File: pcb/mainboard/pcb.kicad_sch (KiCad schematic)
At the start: 28 parts

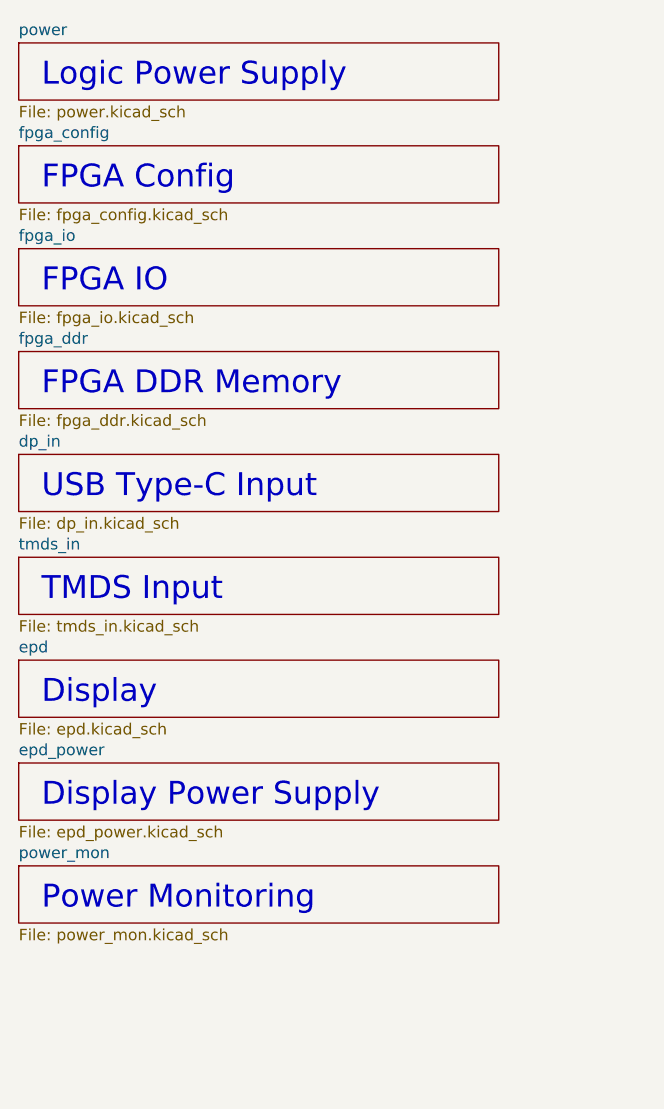
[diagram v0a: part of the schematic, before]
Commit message: PCB r0p10 wip
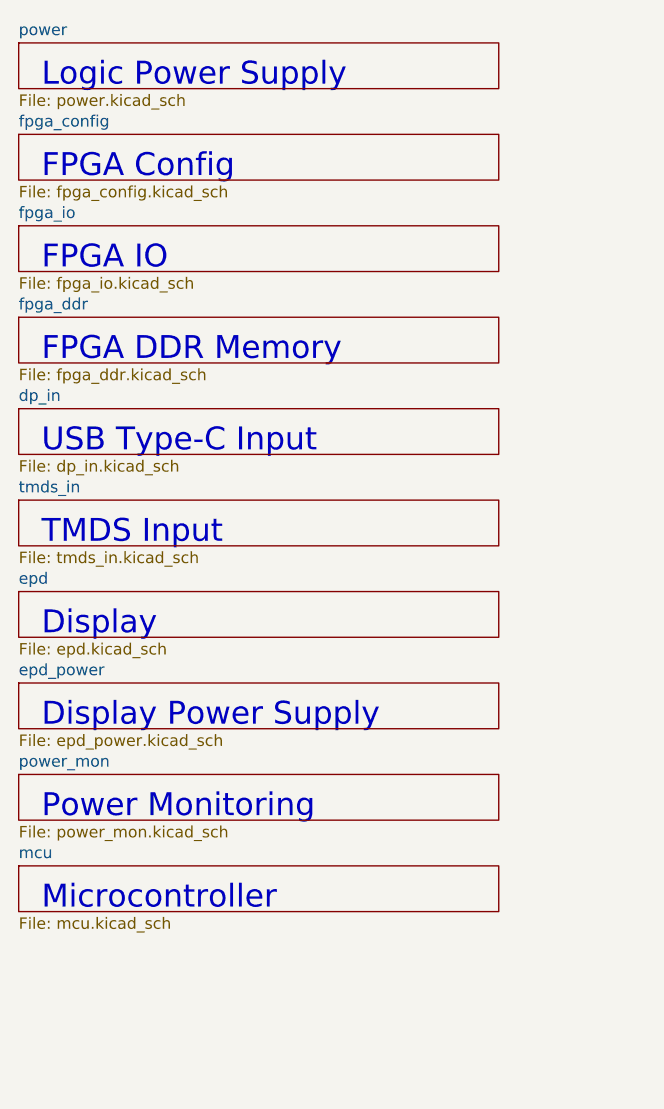
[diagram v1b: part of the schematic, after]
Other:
- added sheet mcu (mcu.kicad_sch)
- note added: "Microcontroller"
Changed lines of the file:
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@@
 	(text "FPGA DDR Memory"
 		(exclude_from_sim no)
-		(at 35.56 67.31 0)
+		(at 35.56 63.5 0)
 		(effects
 			(font
@@
 	(text "Power Monitoring"
 		(exclude_from_sim no)
-		(at 35.56 124.46 0)
+		(at 35.56 114.3 0)
 		(effects
 			(font
@@
 	(text "USB Type-C Input"
 		(exclude_from_sim no)
-		(at 35.56 78.74 0)
+		(at 35.56 73.66 0)
 		(effects
 			(font
@@
 	(text "FPGA Config"
 		(exclude_from_sim no)
-		(at 35.56 44.45 0)
+		(at 35.56 43.18 0)
 		(effects
 			(font
@@
 	(text "Display Power Supply"
 		(exclude_from_sim no)
-		(at 35.56 113.03 0)
+		(at 35.56 104.14 0)
 		(effects
 			(font
@@
 	(text "Display"
 		(exclude_from_sim no)
-		(at 35.56 101.6 0)
+		(at 35.56 93.98 0)
 		(effects
 			(font
@@
 	(text "FPGA IO"
 		(exclude_from_sim no)
-		(at 35.56 55.88 0)
+		(at 35.56 53.34 0)
+		(effects
+			(font
+				(size 2.54 2.54)
+			)
+			(justify left bottom)
+		)
+	)
+	(text "Microcontroller"
+		(exclude_from_sim no)
+		(at 35.56 124.46 0)
 		(effects
 			(font
@@
 	(text "TMDS Input"
 		(exclude_from_sim no)
-		(at 35.56 90.17 0)
+		(at 35.56 83.82 0)
 		(effects
 			(font
@@
 	)
 	(sheet
-		(at 33.02 96.52)
-		(size 53.34 6.35)
+		(at 33.02 88.9)
+		(size 53.34 5.08)
 		(fields_autoplaced yes)
 		(stroke
@@
 		)
 		(property "Sheetname" "epd"
-			(at 33.02 95.8084 0)
+			(at 33.02 88.1884 0)
 			(effects
 				(font
@@
 		)
 		(property "Sheetfile" "epd.kicad_sch"
-			(at 33.02 103.4546 0)
+			(at 33.02 94.5646 0)
 			(effects
 				(font
@@
 	(sheet
 		(at 33.02 27.94)
-		(size 53.34 6.35)
+		(size 53.34 5.08)
 		(fields_autoplaced yes)
 		(stroke
@@
 		)
 		(property "Sheetfile" "power.kicad_sch"
-			(at 33.02 34.8746 0)
+			(at 33.02 33.6046 0)
 			(effects
 				(font
@@
 	)
 	(sheet
-		(at 33.02 119.38)
-		(size 53.34 6.35)
+		(at 33.02 109.22)
+		(size 53.34 5.08)
 		(fields_autoplaced yes)
 		(stroke
@@
 		)
 		(property "Sheetname" "power_mon"
-			(at 33.02 118.6684 0)
+			(at 33.02 108.5084 0)
 			(effects
 				(font
@@
 		)
 		(property "Sheetfile" "power_mon.kicad_sch"
-			(at 33.02 126.3146 0)
+			(at 33.02 114.8846 0)
 			(effects
 				(font
@@
 	)
 	(sheet
-		(at 33.02 85.09)
-		(size 53.34 6.35)
+		(at 33.02 78.74)
+		(size 53.34 5.08)
 		(fields_autoplaced yes)
 		(stroke
@@
 		)
 		(property "Sheetname" "tmds_in"
-			(at 33.02 84.3784 0)
+			(at 33.02 78.0284 0)
 			(effects
 				(font
@@
 		)
 		(property "Sheetfile" "tmds_in.kicad_sch"
-			(at 33.02 92.0246 0)
+			(at 33.02 84.4046 0)
 			(effects
 				(font
@@
 	)
 	(sheet
-		(at 33.02 39.37)
-		(size 53.34 6.35)
+		(at 33.02 119.38)
+		(size 53.34 5.08)
+		(fields_autoplaced yes)
+		(stroke
+			(width 0.1524)
+			(type solid)
+		)
+		(fill
+			(color 0 0 0 0.0000)
+		)
+		(property "Sheetname" "mcu"
+			(at 33.02 118.6684 0)
+			(effects
+				(font
+					(size 1.27 1.27)
+				)
+				(justify left bottom)
+			)
+		)
+		(property "Sheetfile" "mcu.kicad_sch"
+			(at 33.02 125.0446 0)
+			(effects
+				(font
+					(size 1.27 1.27)
+				)
+				(justify left top)
+			)
+		)
+		(instances
+			(project "pcb"
+				(path "/4654897e-3e2f-4522-96c3-20b19803c088"
+					(page "10")
+				)
+			)
+		)
+	)
+	(sheet
+		(at 33.02 38.1)
+		(size 53.34 5.08)
 		(fields_autoplaced yes)
 		(stroke
@@
 		)
 		(property "Sheetname" "fpga_config"
-			(at 33.02 38.6584 0)
+			(at 33.02 37.3884 0)
 			(effects
 				(font
@@
 		)
 		(property "Sheetfile" "fpga_config.kicad_sch"
-			(at 33.02 46.3046 0)
+			(at 33.02 43.7646 0)
 			(effects
 				(font
@@
 	)
 	(sheet
-		(at 33.02 73.66)
-		(size 53.34 6.35)
+		(at 33.02 68.58)
+		(size 53.34 5.08)
 		(fields_autoplaced yes)
 		(stroke
@@
 		)
 		(property "Sheetname" "dp_in"
-			(at 33.02 72.9484 0)
+			(at 33.02 67.8684 0)
 			(effects
 				(font
@@
 		)
 		(property "Sheetfile" "dp_in.kicad_sch"
-			(at 33.02 80.5946 0)
+			(at 33.02 74.2446 0)
 			(effects
 				(font
@@
 	)
 	(sheet
-		(at 33.02 62.23)
-		(size 53.34 6.35)
+		(at 33.02 58.42)
+		(size 53.34 5.08)
 		(fields_autoplaced yes)
 		(stroke
@@
 		)
 		(property "Sheetname" "fpga_ddr"
-			(at 33.02 61.5184 0)
+			(at 33.02 57.7084 0)
 			(effects
 				(font
@@
 		)
 		(property "Sheetfile" "fpga_ddr.kicad_sch"
-			(at 33.02 69.1646 0)
+			(at 33.02 64.0846 0)
 			(effects
 				(font
@@
 	)
 	(sheet
-		(at 33.02 50.8)
-		(size 53.34 6.35)
+		(at 33.02 48.26)
+		(size 53.34 5.08)
 		(fields_autoplaced yes)
 		(stroke
@@
 		)
 		(property "Sheetname" "fpga_io"
-			(at 33.02 50.0884 0)
+			(at 33.02 47.5484 0)
 			(effects
 				(font
@@
 		)
 		(property "Sheetfile" "fpga_io.kicad_sch"
-			(at 33.02 57.7346 0)
+			(at 33.02 53.9246 0)
 			(effects
 				(font
@@
 	)
 	(sheet
-		(at 33.02 107.95)
-		(size 53.34 6.35)
+		(at 33.02 99.06)
+		(size 53.34 5.08)
 		(fields_autoplaced yes)
 		(stroke
@@
 		)
 		(property "Sheetname" "epd_power"
-			(at 33.02 107.2384 0)
+			(at 33.02 98.3484 0)
 			(effects
 				(font
@@
 		)
 		(property "Sheetfile" "epd_power.kicad_sch"
-			(at 33.02 114.8846 0)
+			(at 33.02 104.7246 0)
 			(effects
 				(font
